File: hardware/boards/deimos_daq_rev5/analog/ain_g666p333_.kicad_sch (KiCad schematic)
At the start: 6 parts, among them IC36001 INA826AIDR

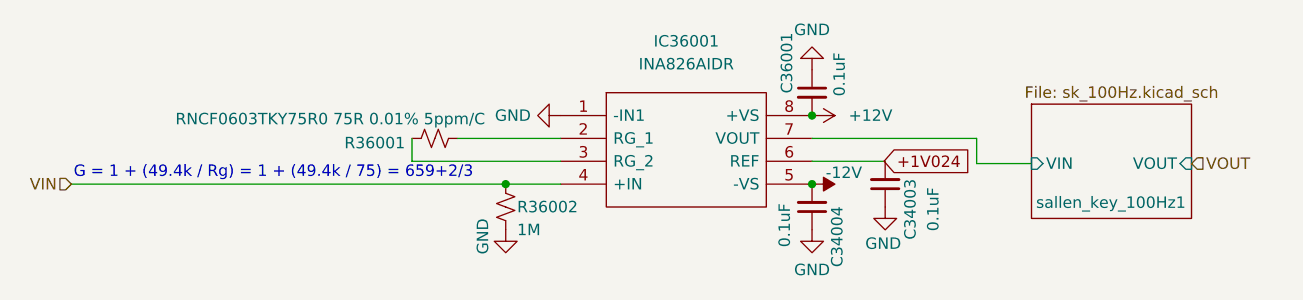
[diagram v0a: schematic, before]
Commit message: restore rev5 and make this rev rev6
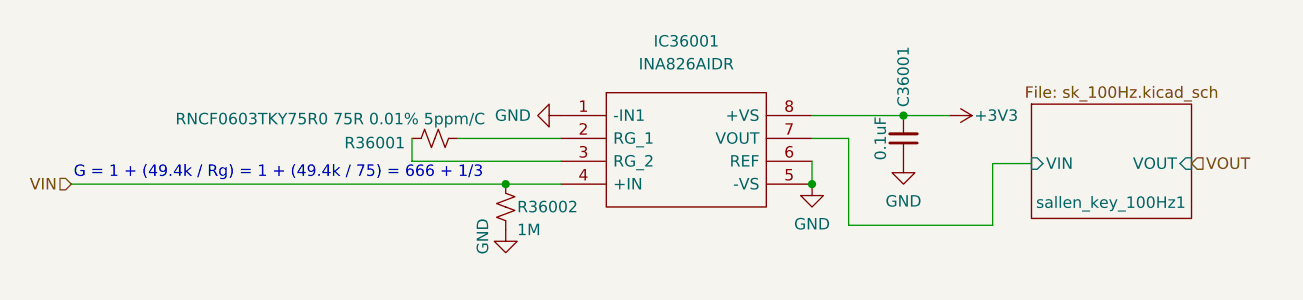
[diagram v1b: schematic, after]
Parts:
- removed C34003, C34004: 0.1uF, Capacitor_SMD:C_0402_1005Metric, symbol Device:C_Small
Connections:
- net +1V024 is gone; now on net GND: IC36001.6 (REF)
- net -12V is gone; now on net GND: IC36001.5 (-VS)
- net +12V renamed +3V3
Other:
- note added: "G = 1 + (49.4k / Rg) = 1 + (49.4k / 75) = 666 + 1/3"
- note removed: "G = 1 + (49.4k / Rg) = 1 + (49.4k / 75) = 659+2/3"
- moved on the sheet: C36001
